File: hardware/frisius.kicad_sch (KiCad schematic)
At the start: 0 parts

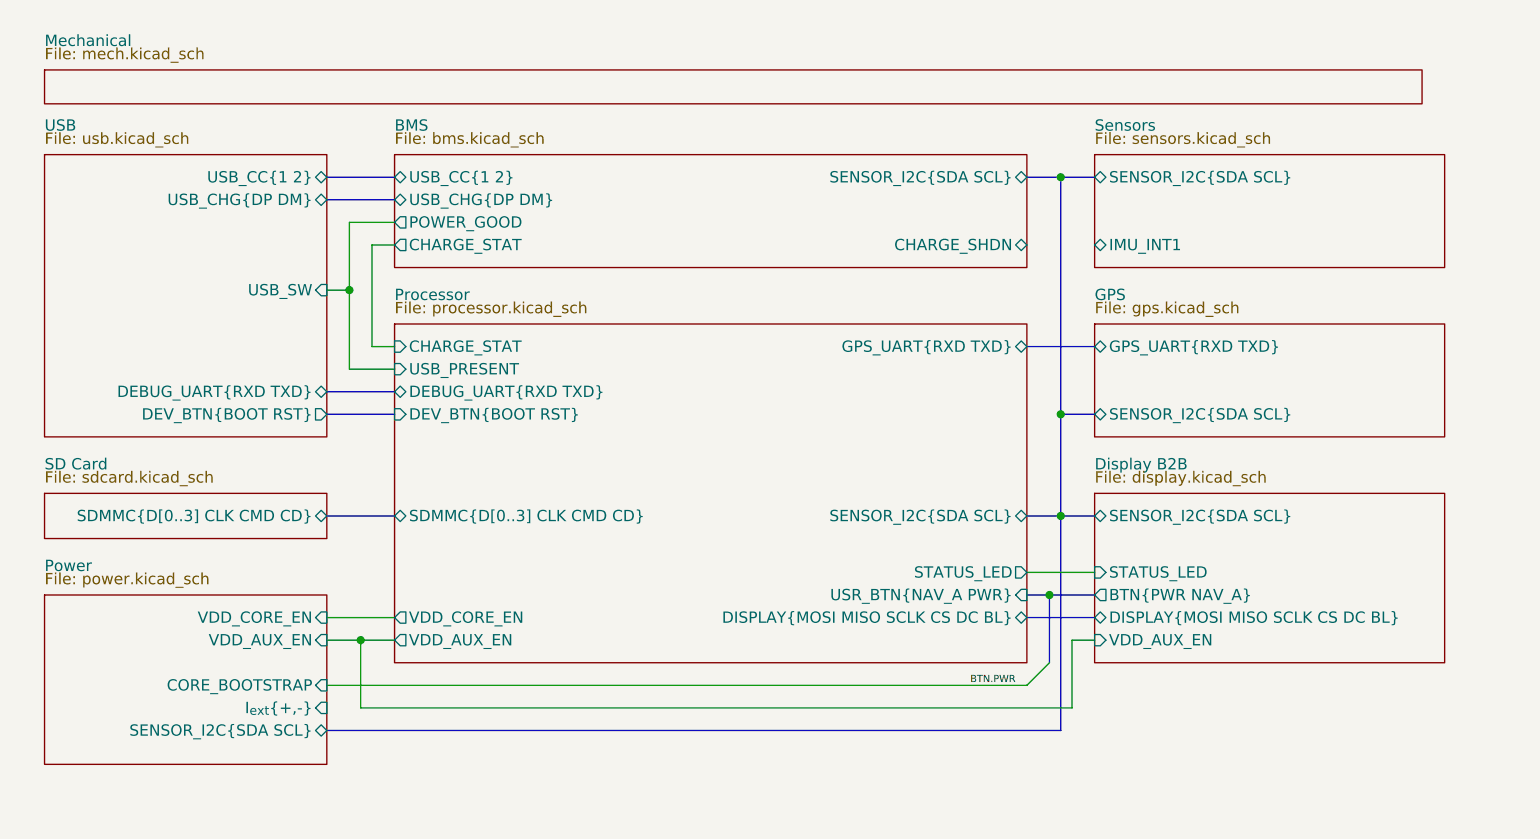
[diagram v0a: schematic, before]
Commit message: hardware update
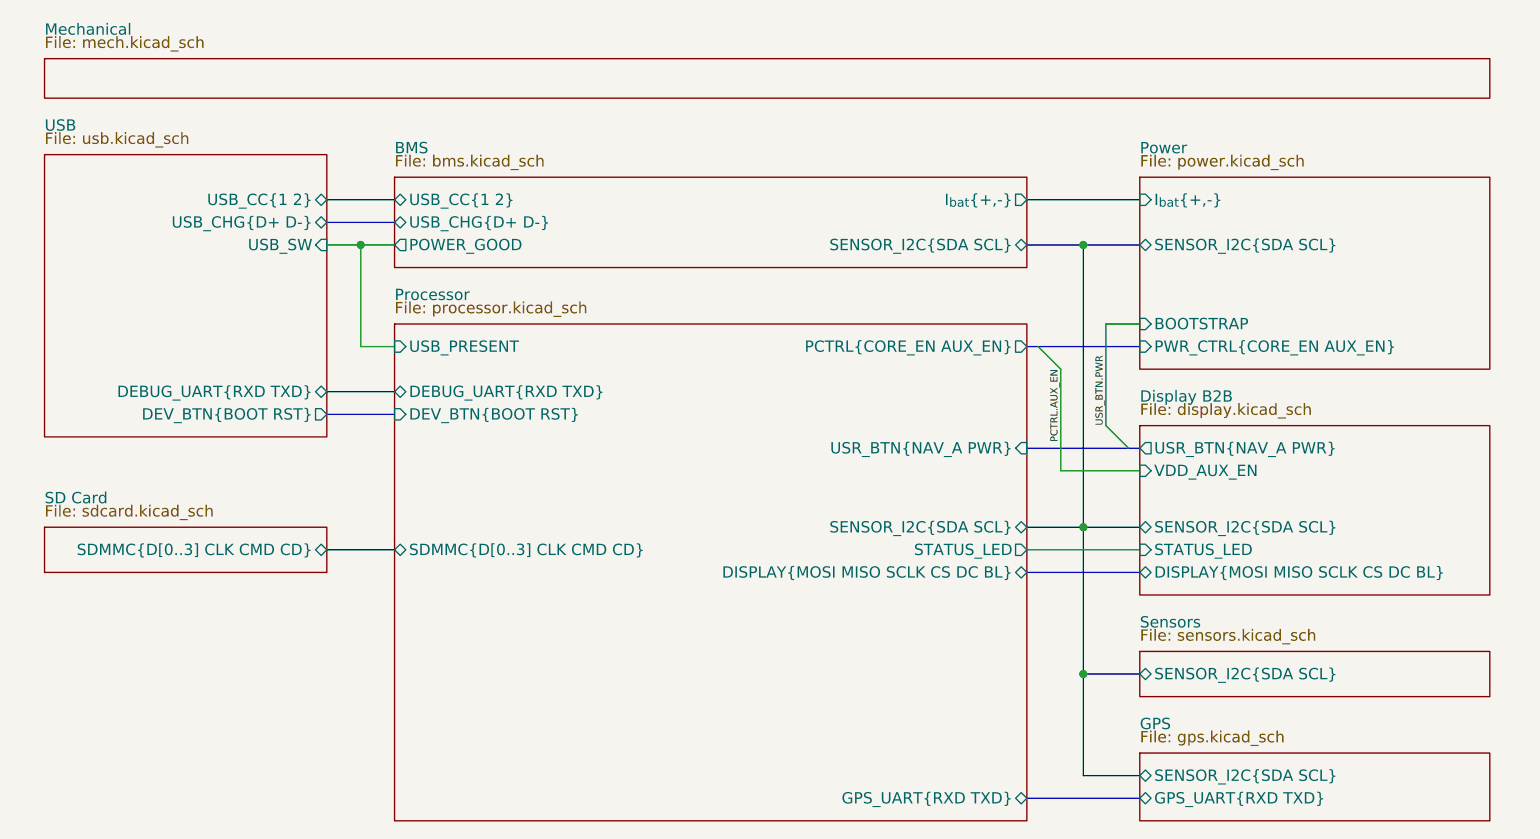
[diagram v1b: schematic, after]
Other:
- sheet BMS ports: added I_{bat}{+,-}, USB_CHG{D+ D-}; removed CHARGE_SHDN, CHARGE_STAT, USB_CHG{DP DM}
- sheet Display B2B ports: added USR_BTN{NAV_A PWR}; removed BTN{PWR NAV_A}
- sheet Power ports: added BOOTSTRAP, I_{bat}{+,-}, PWR_CTRL{CORE_EN AUX_EN}; removed CORE_BOOTSTRAP, I_{ext}{+,-}, VDD_AUX_EN, VDD_CORE_EN
- sheet Processor ports: added PCTRL{CORE_EN AUX_EN}; removed CHARGE_STAT, VDD_AUX_EN, VDD_CORE_EN
- sheet Sensors ports: added none; removed IMU_INT1
- sheet USB ports: added USB_CHG{D+ D-}; removed USB_CHG{DP DM}
